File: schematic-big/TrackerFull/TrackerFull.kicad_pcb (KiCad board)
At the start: 2 copper layers, 43 x 46.9 mm, 57 parts, among them J2 Conn_01x05_Male, J7 Screw_Terminal_01x02, J8 USB_B_Micro, J9 78646-3001, Q1 IRLML5203, Q2 IRLML5203, Q3 IRLML0030, U1 U.FL, U2 LIS3DSH, U3 MCP73831-2-OT, U5 LP2985-3.3, U6 ATtiny85-20SU

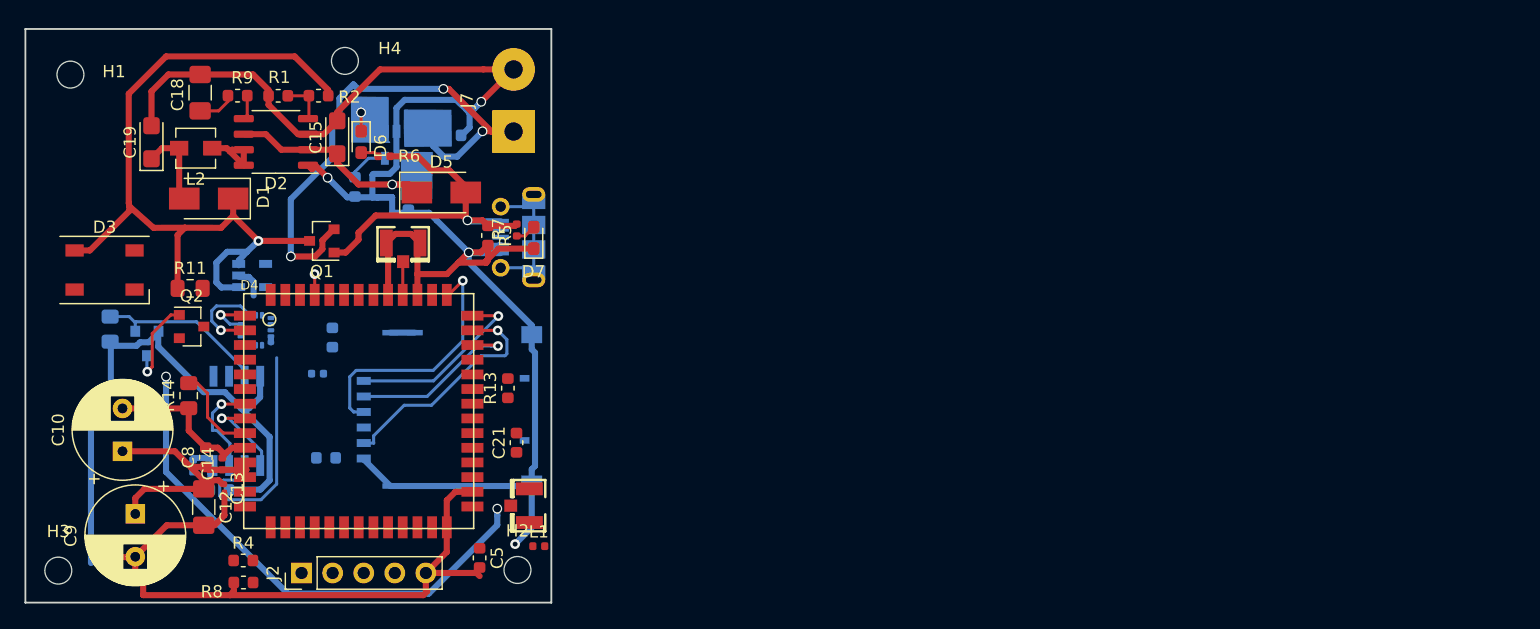
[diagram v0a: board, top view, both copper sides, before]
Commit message: Last schematic
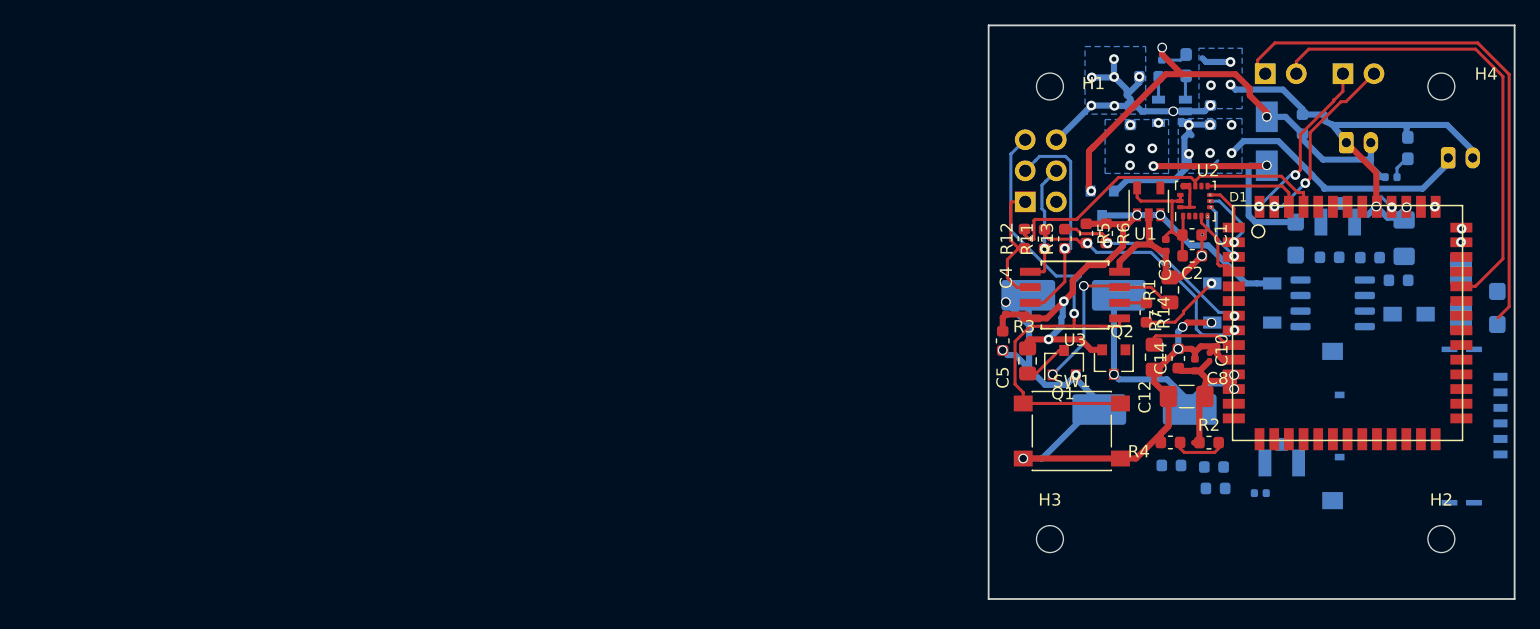
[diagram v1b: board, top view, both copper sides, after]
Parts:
- removed the C14 at (101.3, 101.5)
- removed the C18 at (99.5, 71.2)
- removed C20: 4.7u, Capacitor_SMD:C_0603_1608Metric
- removed C21: 4.7uF, Capacitor_SMD:C_0603_1608Metric
- removed C22: 10uF, Capacitor_SMD:C_0603_1608Metric
- removed the D2 at (105.7, 75.2)
- removed the J2 at (107.8, 110.4)
- removed J8: USB_B_Micro, Connector_USB:USB_Micro-B_Molex-105017-0001
- removed J9: 78646-3001, imported:MOLEX_78646-3001
- removed the R1 at (105.9, 71.4)
- removed the R2 at (109.2, 71.4)
- removed the R3 at (112.1, 78.9)
- removed U6: ATtiny85-20SU, Package_SO:SOIJ-8_5.3x5.3mm_P1.27mm
- added C13: 4.7uF, Capacitor_SMD:C_0603_1608Metric, B.Cu at (182.5, 103.5)
- added C17: 10uF, Capacitor_SMD:C_1206_3216Metric_Pad1.42x1.75mm_HandSolder, B.Cu at (197.9, 83.1)
- added C3: 100nF, Capacitor_SMD:C_0402_1005Metric, F.Cu at (178.4, 83.6)
- added C8: 10pF, Capacitor_SMD:C_0402_1005Metric, F.Cu at (180.8, 93.4)
- added C9: 4.7uF, Capacitor_SMD:C_0603_1608Metric, B.Cu at (178.9, 101.6)
- added D7: D_Schottky, Diode_SMD:D_SMA, B.Cu at (202.6, 87.6)
- added J1: Conn_01x02_Male, Connector_PinHeader_2.54mm:PinHeader_1x02_P2.54mm_Vertical, B.Cu at (186.6, 69.6)
- added J3: AVR-ISP-6, Connector_PinHeader_2.54mm:PinHeader_2x03_P2.54mm_Vertical, B.Cu at (166.9, 80.1)
- added J4: 78646-3001, imported:MOLEX_78646-3001, B.Cu at (198.5, 98.4)
- added J5: Conn_01x02_Male, Connector_PinHeader_2.54mm:PinHeader_1x02_P2.54mm_Vertical, B.Cu at (192.9, 69.6)
- added J6: Screw_Terminal_01x02, Connector_JST:JST_PH_B2B-PH-K_1x02_P2.00mm_Vertical, B.Cu at (193.2, 75.3)
- added R10: 100kOm, Resistor_SMD:R_0603_1608Metric, B.Cu at (189.6, 73.7)
- added R11: 4700, Resistor_SMD:R_0603_1608Metric, F.Cu at (168.5, 83.1)
- added R12: 4700, Resistor_SMD:R_0603_1608Metric, F.Cu at (166.9, 83.1)
- added R15: 250, Resistor_SMD:R_0402_1005Metric, B.Cu at (178.1, 68.0)
- added R16: 100K, Resistor_SMD:R_0603_1608Metric, B.Cu at (182.4, 101.8)
- added R17: 10000, Resistor_SMD:R_0603_1608Metric, B.Cu at (197.4, 86.5)
- added R18: 43000, Resistor_SMD:R_0603_1608Metric, B.Cu at (195.1, 84.7)
- added R19: 10000, Resistor_SMD:R_0603_1608Metric, B.Cu at (191.8, 84.6)
- added R8: 250, Resistor_SMD:R_0402_1005Metric, B.Cu at (196.8, 78.1)
- added SW1: SW_Push, Button_Switch_SMD:SW_Push_1P1T_NO_6x6mm_H9.5mm, F.Cu at (170.7, 98.8)
- added U4: MCP73831-2-OT, Package_TO_SOT_SMD:SOT-23-5, B.Cu at (178.9, 72.7)
- C1: value 10uF -> 4.7u; moved to F.Cu
- C11: renamed from C15; moved to B.Cu
- C15: renamed from C9; footprint Capacitor_THT:CP_Radial_D8.0mm_P3.50mm -> Capacitor_SMD:CP_Elec_8x10.5; moved to B.Cu
- C16: renamed from C10; footprint Capacitor_THT:CP_Radial_D8.0mm_P3.50mm -> Capacitor_SMD:CP_Elec_8x10.5; moved to B.Cu
- C18: renamed from C19; moved to B.Cu
- C2: value 100nF -> 10uF; footprint Capacitor_SMD:C_0402_1005Metric -> Capacitor_SMD:C_0603_1608Metric; moved to F.Cu
- C4: renamed from C23; moved to F.Cu
- C5: value 4.7uF -> 10uF
- D1: value D_Schottky -> A9G; footprint Diode_SMD:D_SMA -> Tracker:A9G2
- D2: renamed from D7; moved to B.Cu
- D3: renamed from D5; moved to B.Cu
- D4: value A9G -> LED; footprint Tracker:A9G2 -> LED_SMD:LED_0603_1608Metric_Pad1.05x0.95mm_HandSolder; moved to B.Cu
- D5: renamed from D3; moved to B.Cu
- D6: value LED -> APW7142; footprint LED_SMD:LED_0603_1608Metric_Pad1.05x0.95mm_HandSolder -> Package_SO:SOP-8_3.9x4.9mm_P1.27mm; moved to B.Cu
- GSM1, L1, L2: moved to B.Cu
- J2: renamed from J7; footprint Connector_Wire:SolderWirePad_1x02_P5.08mm_Drill1.5mm -> Connector_JST:JST_PH_B2B-PH-K_1x02_P2.00mm_Vertical; moved to B.Cu
- Q1: renamed from Q3; moved to F.Cu
- Q3: renamed from Q1; moved to B.Cu
- R1: renamed from R10; moved to F.Cu
- R13: value 100K -> 4700
- R14: value 10K -> 470; footprint Resistor_SMD:R_0805_2012Metric_Pad1.15x1.40mm_HandSolder -> Resistor_SMD:R_0603_1608Metric
- R5: value 100kOm -> 10K
- R6: value 250 -> 10K; footprint Resistor_SMD:R_0402_1005Metric -> Resistor_SMD:R_0603_1608Metric
- R7: value 250 -> 10K; footprint Resistor_SMD:R_0402_1005Metric -> Resistor_SMD:R_0805_2012Metric_Pad1.15x1.40mm_HandSolder
- R9: value 10000 -> 2000; moved to B.Cu
- U1: value U.FL -> LP2985-3.3; footprint mailboxNotifier:U.FL -> Package_TO_SOT_SMD:SOT-23-5
- U2: moved to F.Cu
- U3: value MCP73831-2-OT -> ATtiny85-20SU; footprint Package_TO_SOT_SMD:SOT-23-5 -> Package_SO:SOIJ-8_5.3x5.3mm_P1.27mm; moved to F.Cu
- U5: value LP2985-3.3 -> U.FL; footprint Package_TO_SOT_SMD:SOT-23-5 -> mailboxNotifier:U.FL
- moved C18 110.9 mm to (205.5, 88.8)
- moved L2 100.1 mm to (198.3, 89.3), turned to 0 degrees
- moved D1 93.7 mm to (193.3, 90.0), turned to 0 degrees
- moved D5 93.0 mm to (184.7, 88.4), turned to 180 degrees
- moved H4 89.7 mm to (201.0, 70.7)
- moved R1 86.7 mm to (178.8, 87.3), turned to 90 degrees
- moved U5 85.6 mm to (187.9, 101.4), turned to 90 degrees
- moved C16 83.6 mm to (176.7, 97.1), turned to 180 degrees
- moved C10 81.2 mm to (182.0, 92.8), turned to 90 degrees
- moved H3 81.1 mm to (169.0, 107.7)
- moved C12 80.9 mm to (180.1, 96.0), turned to 180 degrees
- moved D6 80.5 mm to (192.1, 88.4), turned to 0 degrees
- moved H1 80.1 mm to (169.0, 70.7)
- moved C14 79.9 mm to (179.4, 92.9)
- moved R2 79.5 mm to (182.0, 99.8)
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- renumbered C13 to C10, C8 to C14, R4 to R2, R11 to R3, R8 to R4
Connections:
- C1 pad 1: GNDREF -> /3.3v
- C1 pad 2: Net-(C1-Pad2) -> GNDREF
- C2 pad 2: Net-(C1-Pad2) -> /3.3v
- C5 pad 1: /VBAT -> GNDREF
- C5 pad 2: GNDREF -> BAT_IN
- D1 pad 1: BAT_IN -> /ACCEL_CS
- D1 pad 2: /APW_OUT -> /ACCEL_SDO
- D2 pad 2: Net-(D7-Pad2) -> Net-(D2-Pad2)
- D4 pad 1: /ACCEL_SCL -> /CHARGER_STAT
- D4 pad 2: /ACCEL_SDA -> Net-(D4-Pad2)
- D6 pad 1: /CHARGER_STAT -> GNDREF
- D6 pad 2: Net-(D6-Pad2) -> /CHARGER_VDD
- GSM1 pad 3: Net-(D4-Pad45) -> Net-(D1-Pad45)
- R13 pad 1: /VBAT -> /ICSP_SCK
- R13 pad 2: Net-(C21-Pad1) -> /AVR_SCK
- R14 pad 1: GNDREF -> Net-(R14-Pad1)
- R14 pad 2: Net-(D4-Pad9) -> /LED_CTL
- R2 pad 1: /V_BAT -> /VBAT
- R2 pad 2: Net-(D4-Pad15) -> Net-(D1-Pad15)
- R4 pad 1: Net-(D4-Pad15) -> Net-(D1-Pad15)
- R5 pad 1: +5V -> BAT_IN
- R5 pad 2: GNDREF -> /AVR_MOSI_SDA
- R6 pad 1: +5V -> BAT_IN
- R6 pad 2: Net-(D6-Pad2) -> /AVR_SCK
- R7 pad 1: +5V -> GNDREF
- R7 pad 2: Net-(D7-Pad2) -> Net-(D1-Pad9)
- R9 pad 1: Net-(D2-Pad5) -> GNDREF
- R9 pad 2: Net-(C18-Pad2) -> /CHARGER_PROG
- U1 pad 1: GNDREF -> BAT_IN
- U1 pad 3: /GPS_RF -> BAT_IN
- U2 pad 1: Net-(C1-Pad2) -> /3.3v
- U2 pad 14: Net-(C1-Pad2) -> /3.3v
- U2 pad 15: Net-(C1-Pad2) -> /3.3v
- U3 pad 1: /CHARGER_STAT -> /AVR_RST
- U3 pad 2: GNDREF -> Net-(R14-Pad1)
- U3 pad 3: /V_BAT -> /PWR_CTRL
- U3 pad 4: /CHARGER_VDD -> GNDREF
- U3 pad 5: /CHARGER_PROG -> /ICSP_MOSI
- U5 pad 1: BAT_IN -> GNDREF
- U5 pad 3: BAT_IN -> /GPS_RF
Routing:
- net GNDREF: track 272.3 -> 142.9 mm, vias 6 -> 23
- net /HST_RXD: track 0.00 -> 44.0 mm
- net /GPS_RF: track 42.7 -> 0.00 mm, vias 2 -> 0
- net /AVR_RST: track 0.00 -> 42.4 mm, vias 0 -> 1
- net /HST_TXD: track 0.00 -> 38.6 mm
- net /ACCEL_INT1: track 1.70 -> 28.9 mm, vias 1 -> 0
- net BAT_IN: track 70.3 -> 47.5 mm, vias 1 -> 4
- net /SIM_RST: track 21.0 -> 0.00 mm
- net /AVR_MOSI_SDA: track 0.00 -> 20.4 mm, vias 0 -> 2
- net /VSIM: track 19.5 -> 0.00 mm
- net /ICSP_SCK: track 0.00 -> 18.2 mm, vias 0 -> 1
- net /AVR_SCK: track 0.00 -> 17.1 mm, vias 0 -> 2
- net /SIM_CLK: track 15.3 -> 0.00 mm
- net /UART1_RXD: track 0.00 -> 14.8 mm, vias 0 -> 2
- net /SIM_IO: track 14.8 -> 0.00 mm, vias 1 -> 0
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- added copper zone on B.Cu, net /CHARGER_VDD
- added copper zone on B.Cu, net /V_BAT
- added copper zone on B.Cu, net GNDREF
